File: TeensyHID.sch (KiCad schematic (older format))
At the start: 8 parts, among them P1/SCL1 Conn_01x02, P2/SDA1 Conn_01x02, P3/SCL0 Conn_01x02, P4/SDA0 Conn_01x02, SW1 Rotary_Encoder_Switch, SW1POS2 Rotary_Encoder_Switch, SW2 Rotary_Encoder_Switch, U1 Teensy-LC

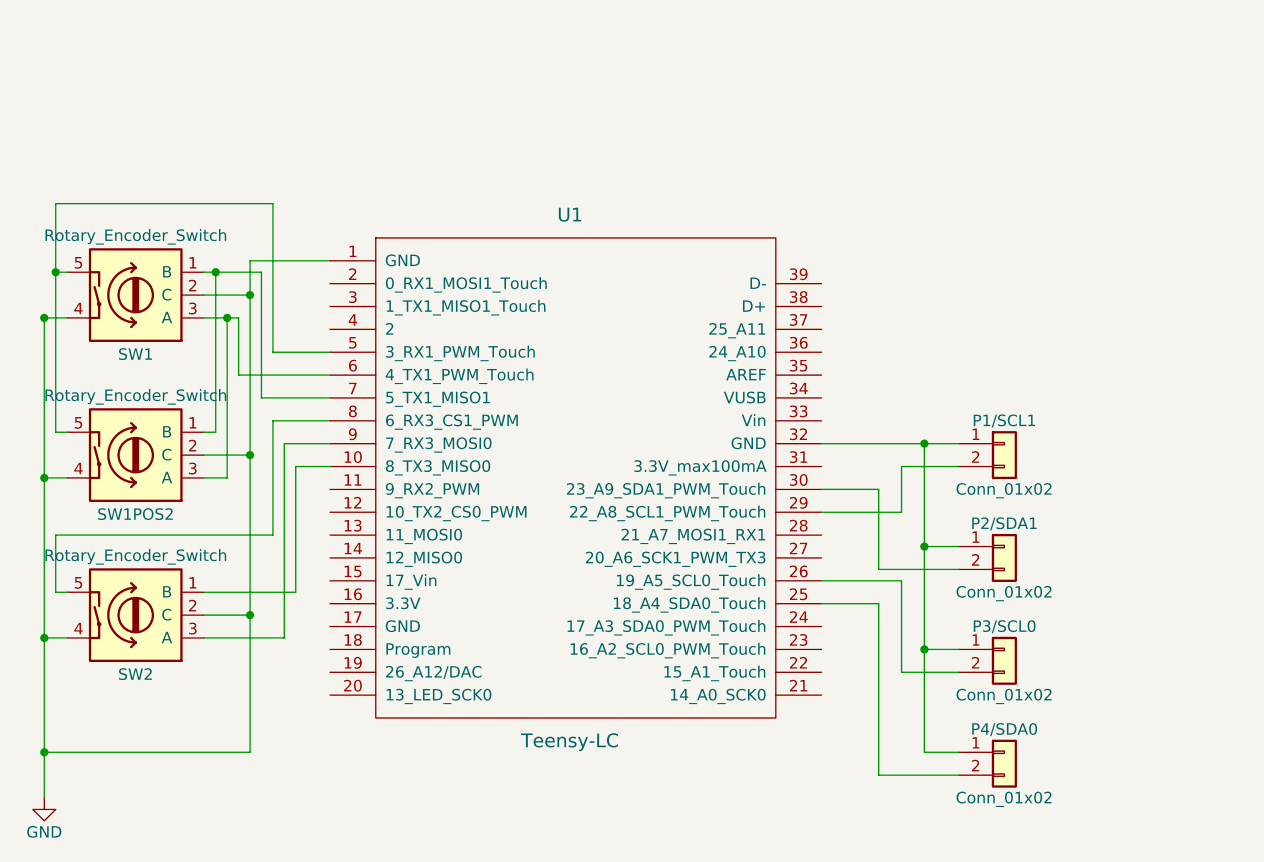
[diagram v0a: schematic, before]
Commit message: 1.1 build of TeensyHID
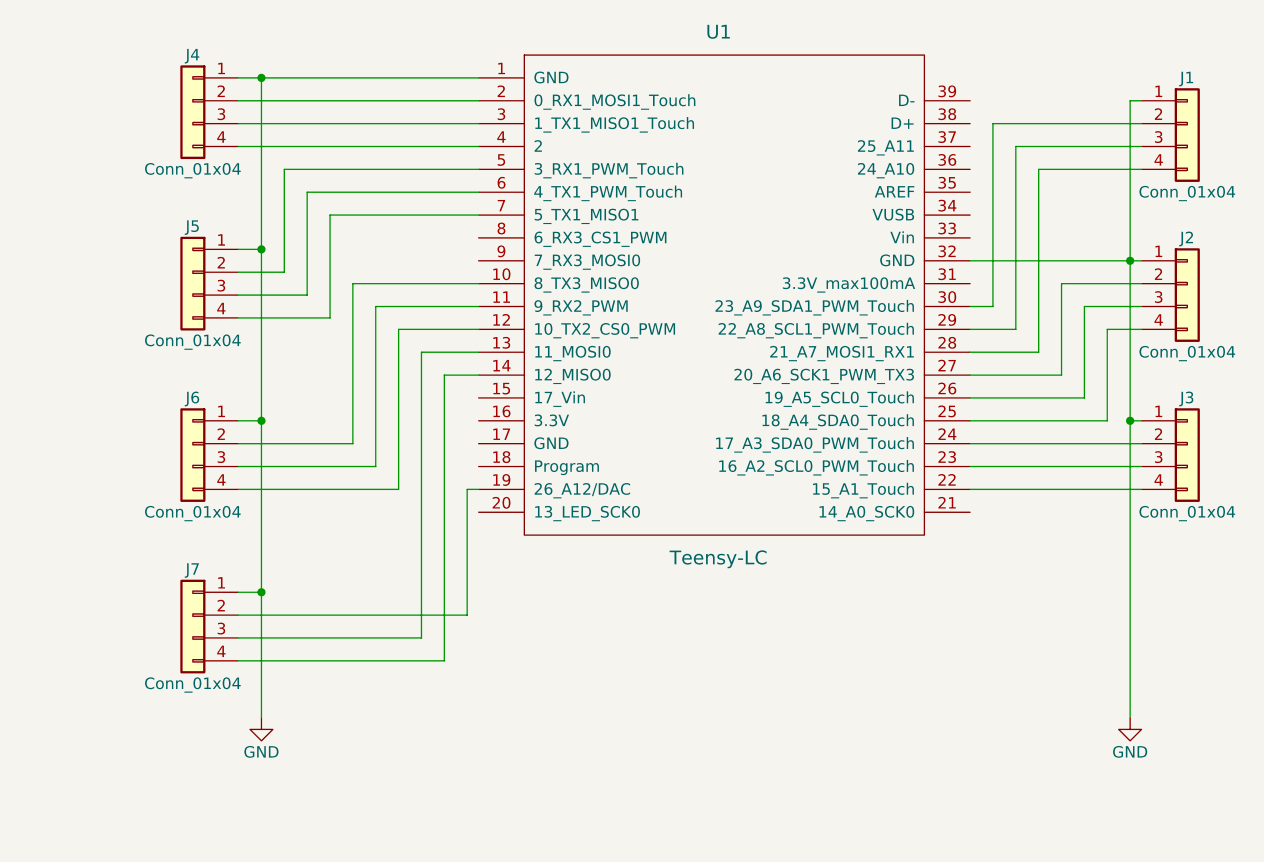
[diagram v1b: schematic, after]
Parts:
- removed P1/SCL1, P2/SDA1, P3/SCL0, P4/SDA0: Conn_01x02, Connectors_JST:JST_EH_B02B-EH-A_02x2.50mm_Straight, symbol Conn_01x02
- removed SW1, SW1POS2, SW2: Rotary_Encoder_Switch, Local Copy:PEC11R-4xxx-Sxxxx, symbol Rotary_Encoder_Switch-RESCUE-TeensyHID
- added J1, J2, J3, J4, J5, J6, J7: Conn_01x04, Connectors_JST:JST_EH_B04B-EH-A_04x2.50mm_Straight, symbol Conn_01x04
- U1: footprint teensy:Teensy30_31_32_LC -> Teensy:Teensy30_31_32_LC
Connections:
- net GND: now also U1.32 (GND), J1.1 (Pin_1), J2.1 (Pin_1), J3.1 (Pin_1), J4.1 (Pin_1), J5.1 (Pin_1), J6.1 (Pin_1), J7.1 (Pin_1)
- net at U1.7 (5_TX1_MISO1): now also J5.4 (Pin_4)
- net at U1.6 (4_TX1_PWM_Touch): now also J5.3 (Pin_3)
- net at U1.5 (3_RX1_PWM_Touch): now also J5.2 (Pin_2)
- net at U1.10 (8_TX3_MISO0): now also J6.2 (Pin_2)
- net at U1.11 (9_RX2_PWM): now also J6.3 (Pin_3)
- net at U1.12 (10_TX2_CS0_PWM): now also J6.4 (Pin_4)
- net at U1.13 (11_MOSI0): now also J7.3 (Pin_3)
- net at U1.14 (12_MISO0): now also J7.4 (Pin_4)
- net at U1.19 (26_A12/DAC): now also J7.2 (Pin_2)
- net at U1.2 (0_RX1_MOSI1_Touch): now also J4.2 (Pin_2)
- net at U1.22 (15_A1_Touch): now also J3.4 (Pin_4)
- net at U1.23 (16_A2_SCL0_PWM_Touch): now also J3.3 (Pin_3)
- net at U1.24 (17_A3_SDA0_PWM_Touch): now also J3.2 (Pin_2)
- net at U1.25 (18_A4_SDA0_Touch): now also J2.4 (Pin_4)
- net at U1.26 (19_A5_SCL0_Touch): now also J2.3 (Pin_3)
- net at U1.27 (20_A6_SCK1_PWM_TX3): now also J2.2 (Pin_2)
- net at U1.28 (21_A7_MOSI1_RX1): now also J1.4 (Pin_4)
- net at U1.29 (22_A8_SCL1_PWM_Touch): now also J1.3 (Pin_3)
- net at U1.3 (1_TX1_MISO1_Touch): now also J4.3 (Pin_3)
- net at U1.30 (23_A9_SDA1_PWM_Touch): now also J1.2 (Pin_2)
- net at U1.4 (2): now also J4.4 (Pin_4)
